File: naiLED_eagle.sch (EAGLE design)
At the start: 11 parts, among them IC1 TCS3414, U2 24LC00T-I/OT, U3 ATTINY85-20SU

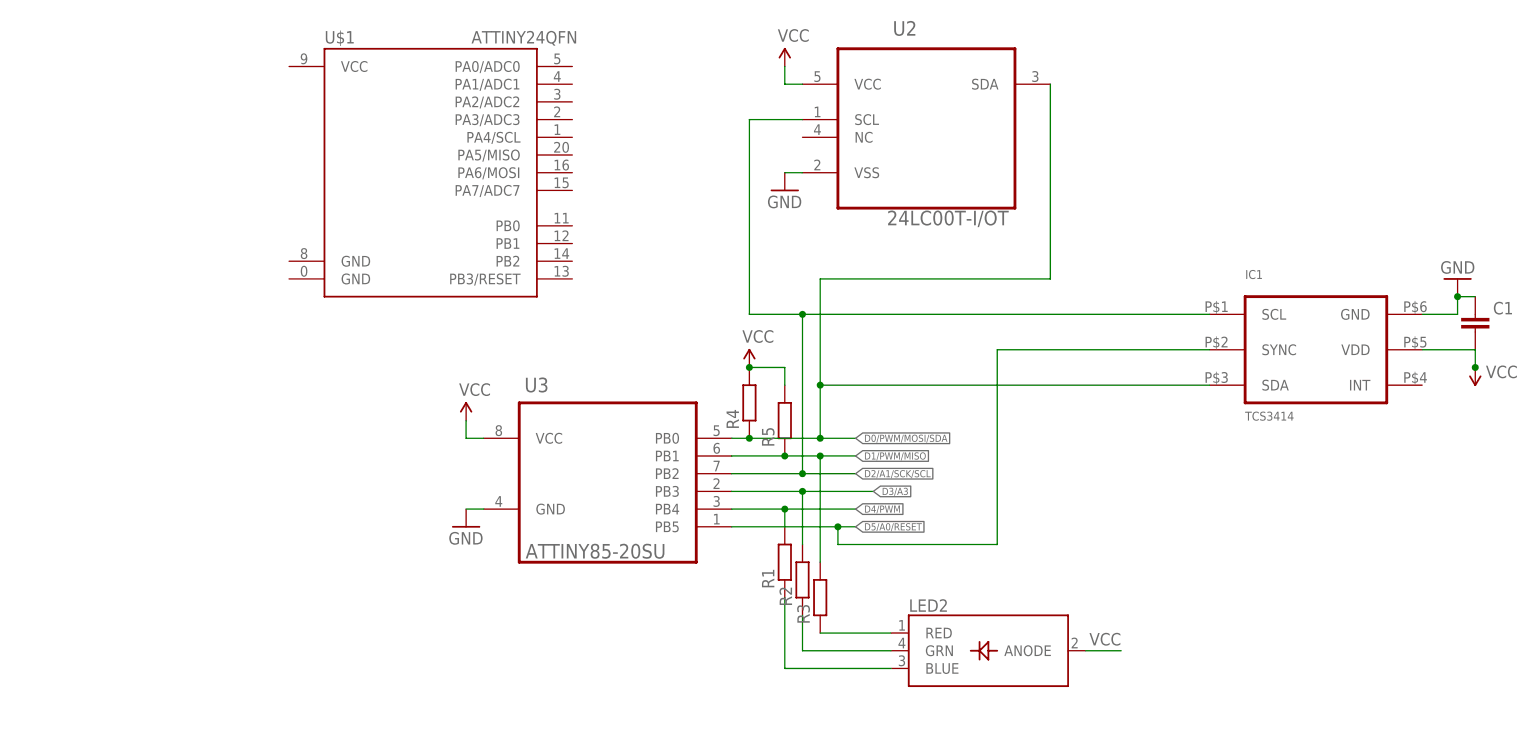
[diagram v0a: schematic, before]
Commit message: working on the at841
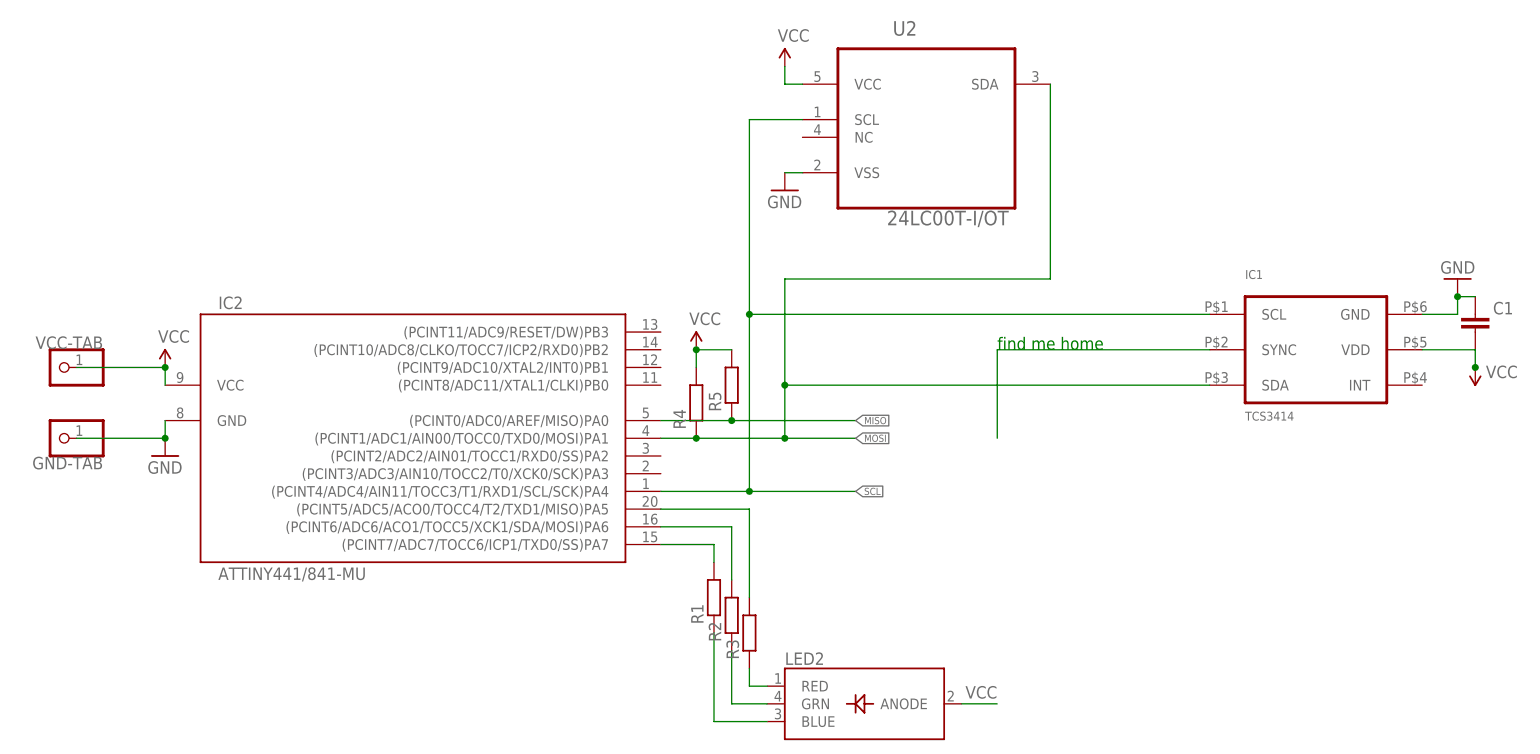
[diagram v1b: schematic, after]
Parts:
- removed U$1: ATTINY24QFN, SparkFun-DigitalIC:ATTINY24QFN
- removed U3: ATTINY85-20SU, nld:ATTINY85-20SU
- added GND-TAB, VCC-TAB: (no value), adafruit:PINHD-1X1CB
- added IC2: ATTINY441/841-MU, nld:ATTINY441/841-MU
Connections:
- removed net D0/PWM/MOSI/SDA: IC1.SDA, R4.1, U2.SDA, U3.PB0
- removed net D1/PWM/MISO: R3.2, R5.1, U3.PB1
- removed net D2/A1/SCK/SCL: IC1.SCL, U2.SCL, U3.PB2
- removed net D3/A3: R2.2, U3.PB3
- removed net D4/PWM: R1.2, U3.PB4
- new net MISO: IC2.(PCINT0/ADC0/AREF/MISO)PA0, R5.1
- new net MOSI: IC1.SDA, IC2.(PCINT1/ADC1/AIN00/TOCC0/TXD0/MOSI)PA1, R4.1, U2.SDA
- new net N$4: IC2.(PCINT7/ADC7/TOCC6/ICP1/TXD0/SS)PA7, R1.2
- new net N$5: IC2.(PCINT6/ADC6/ACO1/TOCC5/XCK1/SDA/MOSI)PA6, R2.2
- new net N$6: IC2.(PCINT5/ADC5/ACO0/TOCC4/T2/TXD1/MISO)PA5, R3.2
- new net SCL: IC1.SCL, IC2.(PCINT4/ADC4/AIN11/TOCC3/T1/RXD1/SCL/SCK)PA4, U2.SCL
- net D5/A0/RESET: no longer U3.PB5
- net GND: now also GND-TAB.1, IC2.GND; no longer U3.GND
- net VCC: now also IC2.VCC, VCC-TAB.1; no longer U3.VCC
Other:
- note added: "find me home"
- moved on the sheet: LED2, R1, R2, R3, R4, R5

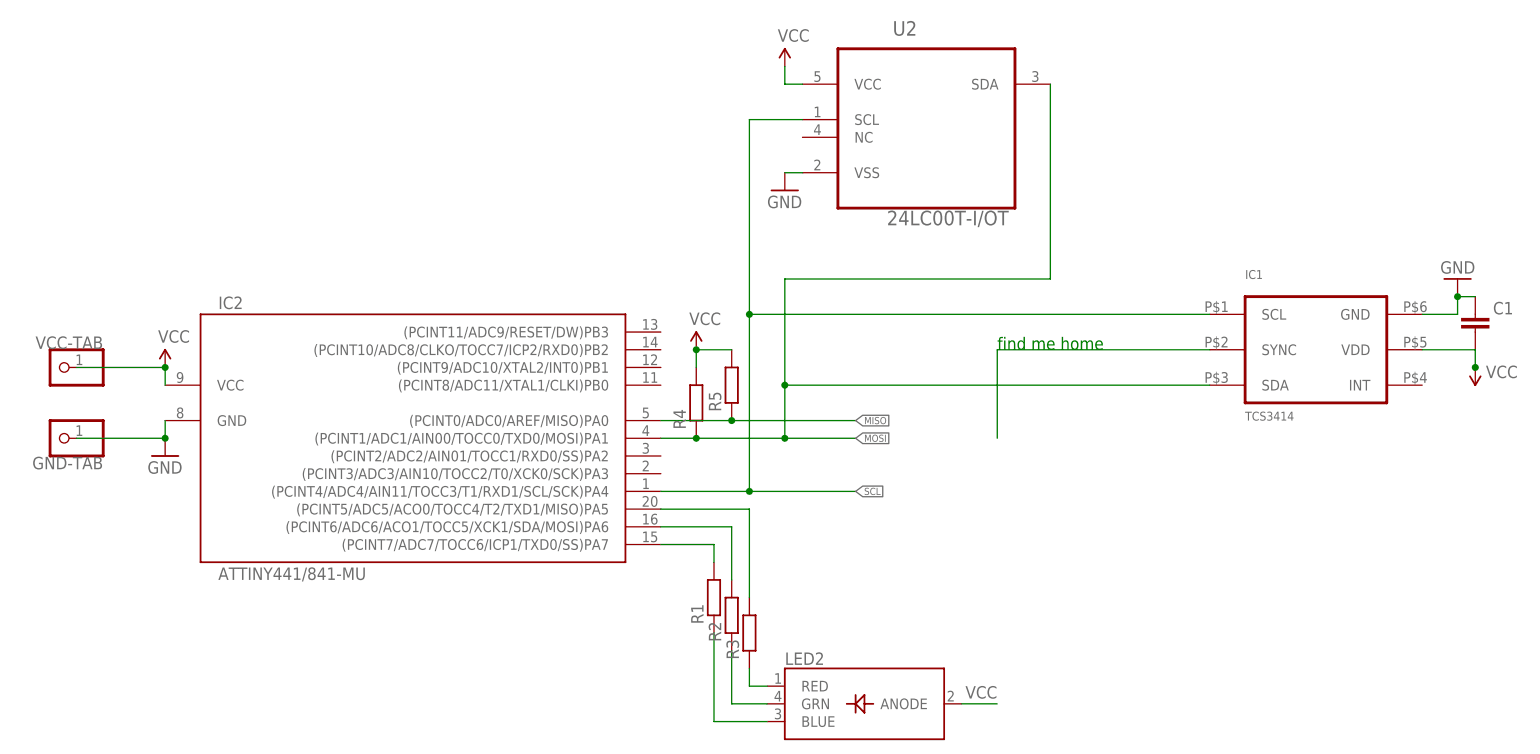
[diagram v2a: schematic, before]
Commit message: some changes, nothing major
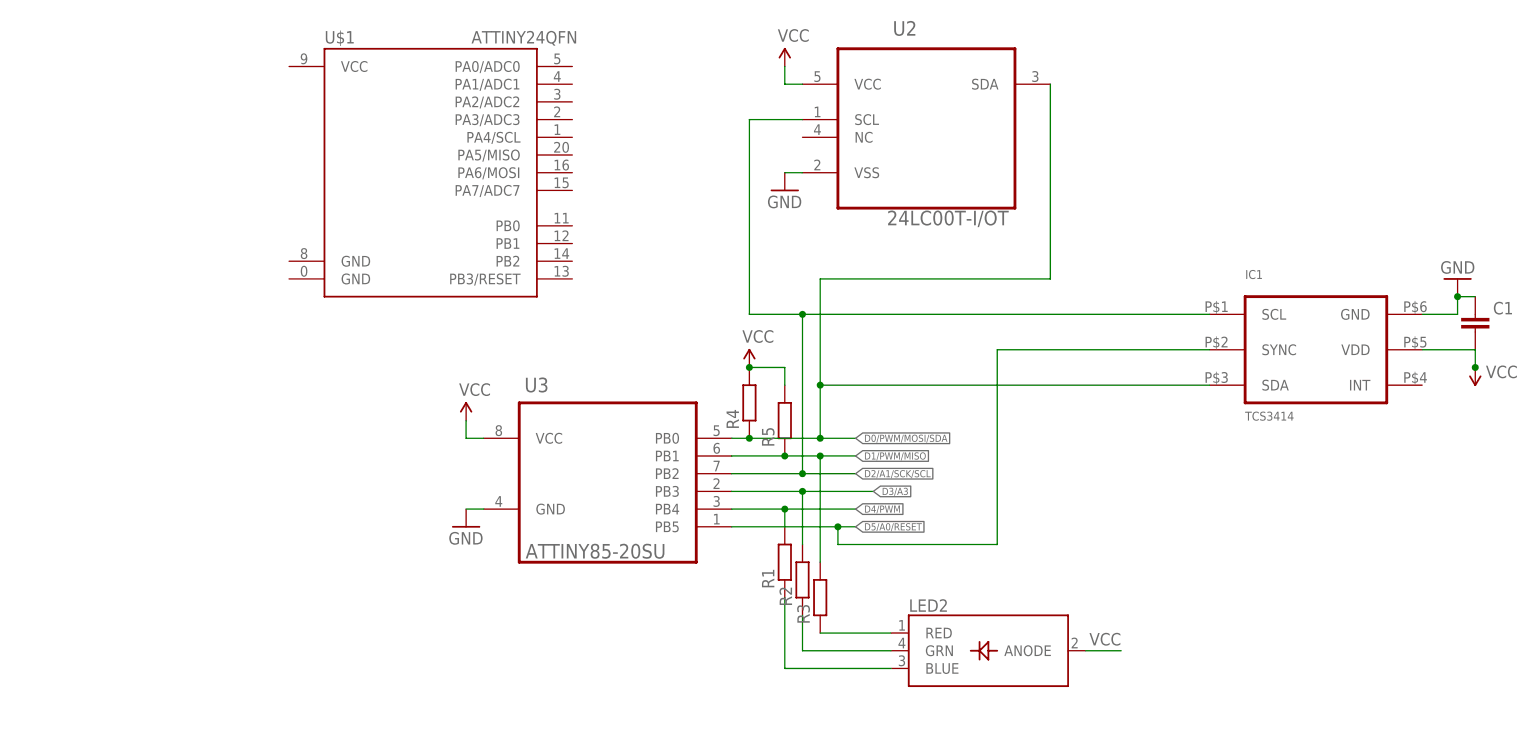
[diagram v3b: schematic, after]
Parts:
- removed GND-TAB, VCC-TAB: (no value), adafruit:PINHD-1X1CB
- removed IC2: ATTINY441/841-MU, nld:ATTINY441/841-MU
- added U$1: ATTINY24QFN, SparkFun-DigitalIC:ATTINY24QFN
- added U3: ATTINY85-20SU, nld:ATTINY85-20SU
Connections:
- removed net MISO: IC2.(PCINT0/ADC0/AREF/MISO)PA0, R5.1
- removed net MOSI: IC1.SDA, IC2.(PCINT1/ADC1/AIN00/TOCC0/TXD0/MOSI)PA1, R4.1, U2.SDA
- removed net N$4: IC2.(PCINT7/ADC7/TOCC6/ICP1/TXD0/SS)PA7, R1.2
- removed net N$5: IC2.(PCINT6/ADC6/ACO1/TOCC5/XCK1/SDA/MOSI)PA6, R2.2
- removed net N$6: IC2.(PCINT5/ADC5/ACO0/TOCC4/T2/TXD1/MISO)PA5, R3.2
- removed net SCL: IC1.SCL, IC2.(PCINT4/ADC4/AIN11/TOCC3/T1/RXD1/SCL/SCK)PA4, U2.SCL
- new net D0/PWM/MOSI/SDA: IC1.SDA, R4.1, U2.SDA, U3.PB0
- new net D1/PWM/MISO: R3.2, R5.1, U3.PB1
- new net D2/A1/SCK/SCL: IC1.SCL, U2.SCL, U3.PB2
- new net D3/A3: R2.2, U3.PB3
- new net D4/PWM: R1.2, U3.PB4
- net D5/A0/RESET: now also U3.PB5
- net GND: now also U3.GND; no longer GND-TAB.1, IC2.GND
- net VCC: now also U3.VCC; no longer IC2.VCC, VCC-TAB.1
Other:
- note removed: "find me home"
- moved on the sheet: LED2, R1, R2, R3, R4, R5
